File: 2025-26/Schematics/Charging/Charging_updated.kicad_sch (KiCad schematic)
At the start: 45 parts, among them J1 DTM04-12PA-L012, J10 Nema 5-20, J11 UPCR012ALS1, J12 UPCP012ALS1, J13 DTM04-12PA-L012, J14 DTM06-12SA, J2 DTM06-12SA, J20 ??? can't find PN, J3 DTM06-12SA, J4 DTM04-12PA-L012, J5 UPCP012ALS2, J6 UPCR012ALS1, J7 DTM04-12PA-L012, J8 DTM06-12SA, J9 J1772, K1 GV24 1BAX, K2 Relay_DPST-NO, K3 P115 BDA, K4 GV24 1BAX, SW1 84-5330.0020, SW2 reset, U12 IMD, U16 Battery Pack, U18 BMS, U19 DS18B20-PAR, U2 Relay board, U20 RSB, U4 6.6kW Elcon Charger, U5 Volt_indic, U6 precharge

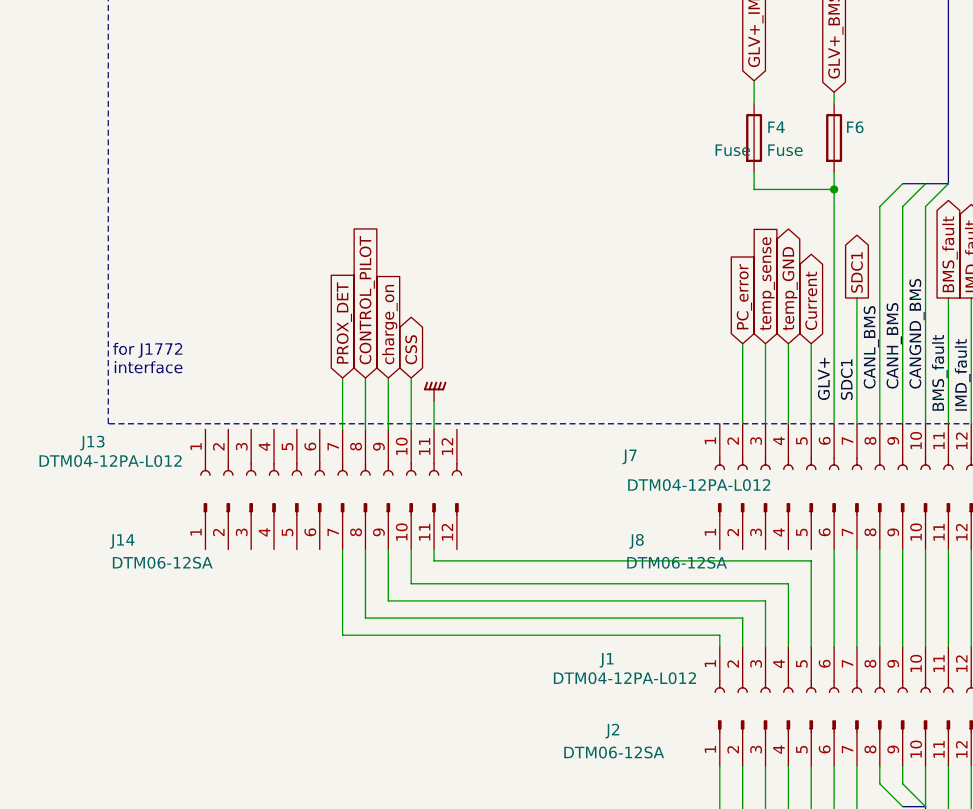
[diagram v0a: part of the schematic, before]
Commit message: Precharge and schematic updates
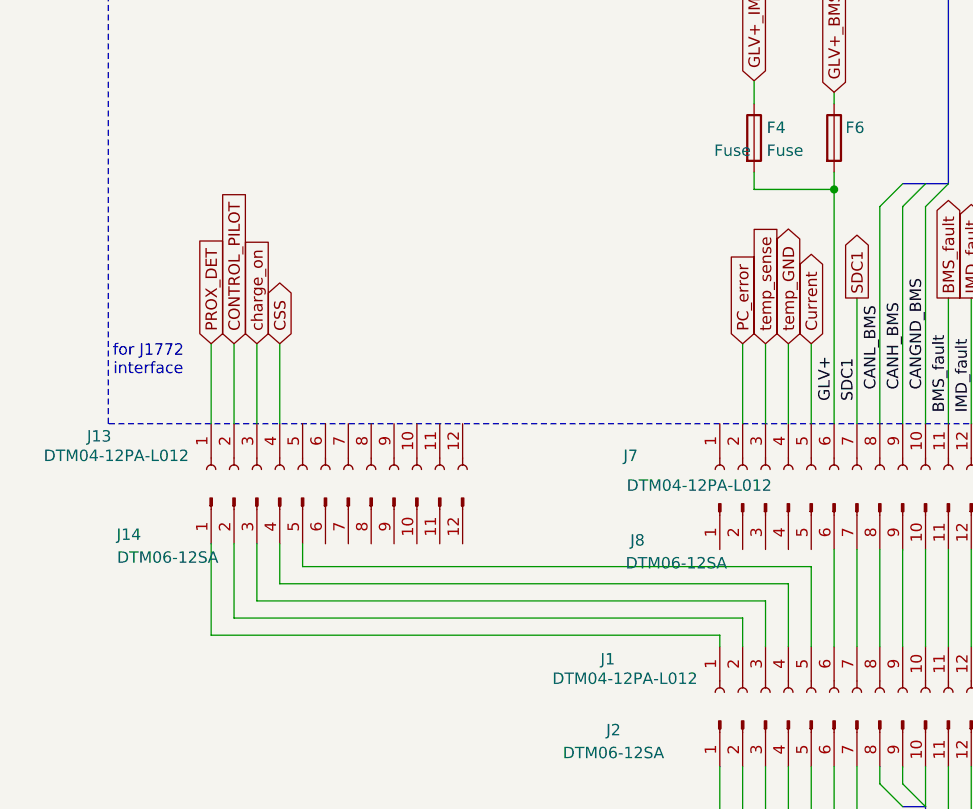
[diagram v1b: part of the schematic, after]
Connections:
- net CONTROL_PILOT: now also J13.2 (Pin_2); no longer J13.8 (Pin_8)
- net CSS: now also J13.4 (Pin_4); no longer J13.10 (Pin_10)
- net GNDPWR: no longer J13.11 (Pin_11)
- net PROX_DET: now also J13.1 (Pin_1); no longer J13.7 (Pin_7)
- net charge_on: now also J13.3 (Pin_3); no longer J13.9 (Pin_9)
- net at U16. (Tap3): no longer U18. (GND_Lug)
- net at J1.1 (Pin_1): now also J14.1 (Pin_1); no longer J14.7 (Pin_7)
- net at J1.2 (Pin_2): now also J14.2 (Pin_2); no longer J14.8 (Pin_8)
- net at J1.3 (Pin_3): now also J14.3 (Pin_3); no longer J14.9 (Pin_9)
- net at J1.4 (Pin_4): now also J14.4 (Pin_4); no longer J14.10 (Pin_10)
- net at J1.5 (Pin_5): now also J14.5 (Pin_5); no longer J14.11 (Pin_11)
- new net: U16. (Tap3), U18. (GND_Lug) (x4)
- now unconnected: U16. (Tap3), U16. (Tap3), U16. (Tap3)
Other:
- moved on the sheet: J13, J14
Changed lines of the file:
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@@
 	(wire
 		(pts
+			(xy 116.205 198.12) (xy 116.205 207.01)
+		)
+		(stroke
+			(width 0)
+			(type default)
+		)
+	)
+	(wire
+		(pts
 			(xy 302.895 153.67) (xy 325.755 153.67)
 		)
@@
 	(wire
 		(pts
-			(xy 135.89 220.98) (xy 135.89 226.695)
+			(xy 121.285 220.345) (xy 121.285 226.695)
 		)
 		(stroke
@@
 	(wire
 		(pts
-			(xy 180.34 224.79) (xy 138.43 224.79)
+			(xy 180.34 224.79) (xy 123.825 224.79)
 		)
 		(stroke
@@
 	(wire
 		(pts
-			(xy 140.97 204.47) (xy 140.97 207.645)
-		)
-		(stroke
-			(width 0)
-			(type default)
-		)
-	)
-	(wire
-		(pts
 			(xy 195.58 284.48) (xy 195.58 313.69)
 		)
@@
 	(wire
 		(pts
-			(xy 130.81 220.98) (xy 130.81 230.505)
+			(xy 116.205 220.345) (xy 116.205 230.505)
 		)
 		(stroke
@@
 	(wire
 		(pts
-			(xy 138.43 201.93) (xy 138.43 207.645)
-		)
-		(stroke
-			(width 0)
-			(type default)
-		)
-	)
-	(wire
-		(pts
 			(xy 253.365 95.885) (xy 270.51 95.885)
 		)
@@
 	(wire
 		(pts
-			(xy 175.26 228.6) (xy 133.35 228.6)
+			(xy 175.26 228.6) (xy 118.745 228.6)
 		)
 		(stroke
@@
 	(wire
 		(pts
-			(xy 138.43 220.98) (xy 138.43 224.79)
+			(xy 123.825 220.345) (xy 123.825 224.79)
 		)
 		(stroke
@@
 	(wire
 		(pts
-			(xy 140.97 220.98) (xy 140.97 222.25)
+			(xy 126.365 220.345) (xy 126.365 222.885)
 		)
 		(stroke
@@
 	(wire
 		(pts
+			(xy 118.745 198.12) (xy 118.745 207.01)
+		)
+		(stroke
+			(width 0)
+			(type default)
+		)
+	)
+	(wire
+		(pts
 			(xy 178.435 48.26) (xy 179.07 48.26)
 		)
@@
 	(wire
 		(pts
-			(xy 133.35 201.93) (xy 133.35 207.645)
-		)
-		(stroke
-			(width 0)
-			(type default)
-		)
-	)
-	(wire
-		(pts
 			(xy 180.34 284.48) (xy 180.34 287.02)
 		)
@@
 	(wire
 		(pts
+			(xy 123.825 198.12) (xy 123.825 207.01)
+		)
+		(stroke
+			(width 0)
+			(type default)
+		)
+	)
+	(wire
+		(pts
 			(xy 172.72 230.505) (xy 172.72 231.775)
 		)
@@
 	(wire
 		(pts
-			(xy 140.97 222.25) (xy 182.88 222.25)
+			(xy 126.365 222.885) (xy 182.88 222.885)
 		)
 		(stroke
@@
 	(wire
 		(pts
+			(xy 121.285 198.12) (xy 121.285 207.01)
+		)
+		(stroke
+			(width 0)
+			(type default)
+		)
+	)
+	(wire
+		(pts
 			(xy 204.47 88.9) (xy 204.47 63.5)
 		)
@@
 	(wire
 		(pts
-			(xy 135.89 201.93) (xy 135.89 207.645)
-		)
-		(stroke
-			(width 0)
-			(type default)
-		)
-	)
-	(wire
-		(pts
 			(xy 375.92 97.79) (xy 384.81 97.79)
 		)
@@
 	(wire
 		(pts
-			(xy 130.81 201.93) (xy 130.81 207.645)
-		)
-		(stroke
-			(width 0)
-			(type default)
-		)
-	)
-	(wire
-		(pts
 			(xy 393.065 374.65) (xy 395.605 374.65)
 		)
@@
 	(wire
 		(pts
-			(xy 135.89 226.695) (xy 177.8 226.695)
+			(xy 121.285 226.695) (xy 177.8 226.695)
 		)
 		(stroke
@@
 	(wire
 		(pts
-			(xy 182.88 222.25) (xy 182.88 231.775)
+			(xy 182.88 222.885) (xy 182.88 231.775)
 		)
 		(stroke
@@
 	(wire
 		(pts
-			(xy 130.81 230.505) (xy 172.72 230.505)
+			(xy 116.205 230.505) (xy 172.72 230.505)
 		)
 		(stroke
@@
 	(wire
 		(pts
-			(xy 133.35 228.6) (xy 133.35 220.98)
+			(xy 118.745 228.6) (xy 118.745 220.345)
 		)
 		(stroke
@@
 	(global_label "charge_on"
 		(shape input)
-		(at 135.89 201.93 90)
+		(at 121.285 198.12 90)
 		(fields_autoplaced yes)
 		(effects
@@
 		)
 		(property "Intersheetrefs" "${INTERSHEET_REFS}"
-			(at 135.89 189.2688 90)
+			(at 121.285 185.4588 90)
 			(effects
 				(font
@@
 	(global_label "CONTROL_PILOT"
 		(shape input)
-		(at 133.35 201.93 90)
+		(at 118.745 198.12 90)
 		(fields_autoplaced yes)
 		(effects
@@
 		)
 		(property "Intersheetrefs" "${INTERSHEET_REFS}"
-			(at 133.35 184.249 90)
+			(at 118.745 180.439 90)
 			(effects
 				(font
@@
 	(global_label "PROX_DET"
 		(shape input)
-		(at 130.81 201.93 90)
+		(at 116.205 198.12 90)
 		(fields_autoplaced yes)
 		(effects
@@
 		)
 		(property "Intersheetrefs" "${INTERSHEET_REFS}"
-			(at 130.81 189.5106 90)
+			(at 116.205 185.7006 90)
 			(effects
 				(font
@@
 	(global_label "CSS"
 		(shape bidirectional)
-		(at 138.43 201.93 90)
+		(at 123.825 198.12 90)
 		(fields_autoplaced yes)
 		(effects
@@
 		)
 		(property "Intersheetrefs" "${INTERSHEET_REFS}"
-			(at 138.43 194.1445 90)
+			(at 123.825 190.3345 90)
 			(effects
 				(font
@@
 	(symbol
 		(lib_id "Connector:Conn_01x12_Socket")
-		(at 128.27 212.725 90)
+		(at 128.905 212.09 90)
 		(mirror x)
 		(unit 1)
@@
 		(dnp no)
 		(property "Reference" "J13"
-			(at 103.124 209.042 90)
+			(at 103.759 208.407 90)
 			(effects
 				(font
@@
 		)
 		(property "Value" "DTM04-12PA-L012"
-			(at 105.029 211.201 90)
+			(at 105.664 210.566 90)
 			(effects
 				(font
@@
 		)
 		(property "Footprint" ""
-			(at 128.27 212.725 0)
+			(at 128.905 212.09 0)
 			(effects
 				(font
@@
 		)
 		(property "Datasheet" "~"
-			(at 128.27 212.725 0)
+			(at 128.905 212.09 0)
 			(effects
 				(font
@@
 		)
 		(property "Description" ""
-			(at 128.27 212.725 0)
+			(at 128.905 212.09 0)
 			(effects
 				(font
@@
 	)
 	(symbol
-		(lib_id "power:GNDPWR")
-		(at 140.97 204.47 180)
-		(unit 1)
-		(exclude_from_sim no)
-		(in_bom yes)
-		(on_board yes)
-		(dnp no)
-		(fields_autoplaced yes)
-		(property "Reference" "#PWR09"
-			(at 140.97 199.39 0)
-			(effects
-				(font
-					(size 1.27 1.27)
-				)
-				(hide yes)
-			)
-		)
-		(property "Value" "GNDPWR"
-			(at 141.097 200.66 0)
-			(effects
-				(font
-					(size 1.27 1.27)
-				)
-				(hide yes)
-			)
-		)
-		(property "Footprint" ""
-			(at 140.97 203.2 0)
-			(effects
-				(font
-					(size 1.27 1.27)
-				)
-				(hide yes)
-			)
-		)
-		(property "Datasheet" ""
-			(at 140.97 203.2 0)
-			(effects
-				(font
-					(size 1.27 1.27)
-				)
-				(hide yes)
-			)
-		)
-		(property "Description" "Power symbol creates a global label with name \"GNDPWR\" , global ground"
-			(at 140.97 204.47 0)
-			(effects
-				(font
-					(size 1.27 1.27)
-				)
-				(hide yes)
-			)
-		)
-		(pin "1"
-		)
-		(instances
-			(project "Charging_updated"
-				(path "/37f4dd62-26e6-4f3a-ae02-c1fd86435617"
-					(reference "#PWR09")
-					(unit 1)
-				)
-			)
-		)
-	)
-	(symbol
 		(lib_id "Connector:Conn_01x04_Socket")
 		(at 221.615 106.68 0)
@@
 	(symbol
 		(lib_id "Connector:Conn_01x12_Pin")
-		(at 128.27 215.9 90)
+		(at 128.905 215.265 90)
 		(mirror x)
 		(unit 1)
@@
 		(dnp no)
 		(property "Reference" "J14"
-			(at 106.426 219.964 90)
+			(at 107.061 219.329 90)
 			(effects
 				(font
@@
 		)
 		(property "Value" "DTM06-12SA"
-			(at 110.744 222.504 90)
+			(at 111.379 221.869 90)
 			(effects
 				(font
@@
 		)
 		(property "Footprint" ""
-			(at 128.27 215.9 0)
+			(at 128.905 215.265 0)
 			(effects
 				(font
@@
 		)
 		(property "Datasheet" "~"
-			(at 128.27 215.9 0)
+			(at 128.905 215.265 0)
 			(effects
 				(font
@@
 		)
 		(property "Description" ""
-			(at 128.27 215.9 0)
+			(at 128.905 215.265 0)
 			(effects
 				(font

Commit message: Precharge board updates and schematic changes
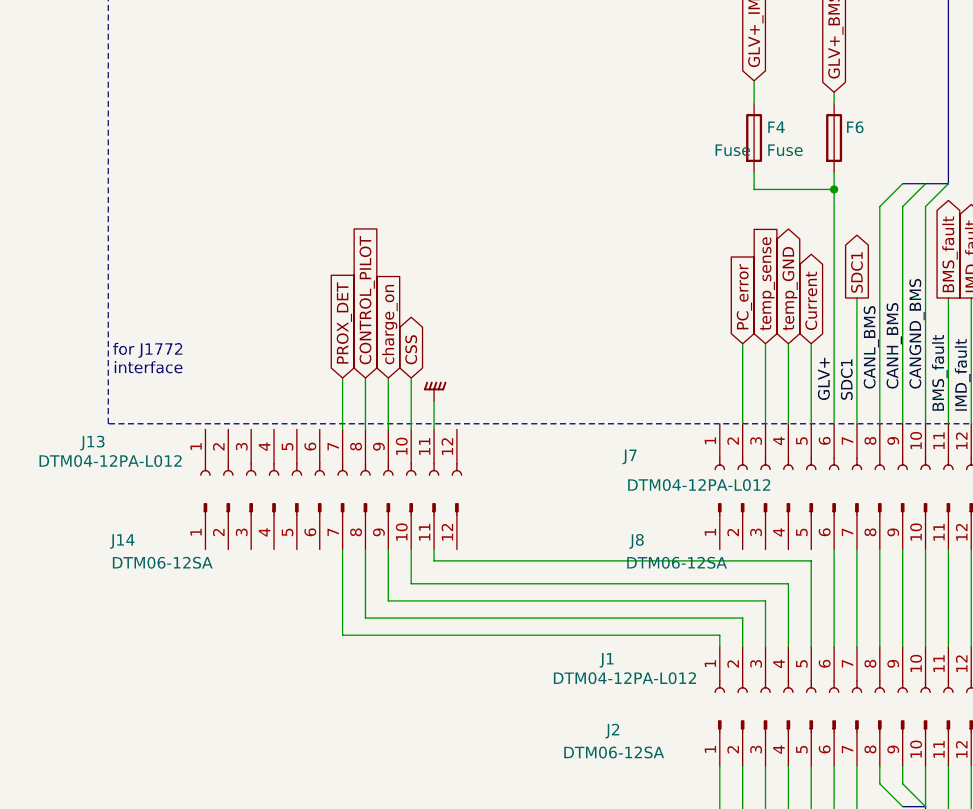
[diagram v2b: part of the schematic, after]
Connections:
- net CONTROL_PILOT: now also J13.8 (Pin_8); no longer J13.2 (Pin_2)
- net CSS: now also J13.10 (Pin_10); no longer J13.4 (Pin_4)
- net GNDPWR: now also J13.11 (Pin_11)
- net PROX_DET: now also J13.7 (Pin_7); no longer J13.1 (Pin_1)
- net charge_on: now also J13.9 (Pin_9); no longer J13.3 (Pin_3)
- net at U16. (Tap3): no longer U18. (GND_Lug)
- net at J1.1 (Pin_1): now also J14.7 (Pin_7); no longer J14.1 (Pin_1)
- net at J1.2 (Pin_2): now also J14.8 (Pin_8); no longer J14.2 (Pin_2)
- net at J1.3 (Pin_3): now also J14.9 (Pin_9); no longer J14.3 (Pin_3)
- net at J1.4 (Pin_4): now also J14.10 (Pin_10); no longer J14.4 (Pin_4)
- net at J1.5 (Pin_5): now also J14.11 (Pin_11); no longer J14.5 (Pin_5)
- new net: U16. (Tap3), U18. (GND_Lug) (x4)
- now unconnected: U16. (Tap3), U16. (Tap3), U16. (Tap3)
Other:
- moved on the sheet: J13, J14
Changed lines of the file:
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@@
 	(wire
 		(pts
-			(xy 116.205 198.12) (xy 116.205 207.01)
-		)
-		(stroke
-			(width 0)
-			(type default)
-		)
-	)
-	(wire
-		(pts
 			(xy 302.895 153.67) (xy 325.755 153.67)
 		)
@@
 	(wire
 		(pts
-			(xy 121.285 220.345) (xy 121.285 226.695)
+			(xy 135.89 220.98) (xy 135.89 226.695)
 		)
 		(stroke
@@
 	(wire
 		(pts
-			(xy 180.34 224.79) (xy 123.825 224.79)
+			(xy 180.34 224.79) (xy 138.43 224.79)
 		)
 		(stroke
@@
 	(wire
 		(pts
+			(xy 140.97 204.47) (xy 140.97 207.645)
+		)
+		(stroke
+			(width 0)
+			(type default)
+		)
+	)
+	(wire
+		(pts
 			(xy 195.58 284.48) (xy 195.58 313.69)
 		)
@@
 	(wire
 		(pts
-			(xy 116.205 220.345) (xy 116.205 230.505)
+			(xy 130.81 220.98) (xy 130.81 230.505)
 		)
 		(stroke
@@
 	(wire
 		(pts
+			(xy 138.43 201.93) (xy 138.43 207.645)
+		)
+		(stroke
+			(width 0)
+			(type default)
+		)
+	)
+	(wire
+		(pts
 			(xy 253.365 95.885) (xy 270.51 95.885)
 		)
@@
 	(wire
 		(pts
-			(xy 175.26 228.6) (xy 118.745 228.6)
+			(xy 175.26 228.6) (xy 133.35 228.6)
 		)
 		(stroke
@@
 	(wire
 		(pts
-			(xy 123.825 220.345) (xy 123.825 224.79)
+			(xy 138.43 220.98) (xy 138.43 224.79)
 		)
 		(stroke
@@
 	(wire
 		(pts
-			(xy 126.365 220.345) (xy 126.365 222.885)
+			(xy 140.97 220.98) (xy 140.97 222.25)
 		)
 		(stroke
@@
 	(wire
 		(pts
-			(xy 118.745 198.12) (xy 118.745 207.01)
-		)
-		(stroke
-			(width 0)
-			(type default)
-		)
-	)
-	(wire
-		(pts
 			(xy 178.435 48.26) (xy 179.07 48.26)
 		)
@@
 	(wire
 		(pts
+			(xy 133.35 201.93) (xy 133.35 207.645)
+		)
+		(stroke
+			(width 0)
+			(type default)
+		)
+	)
+	(wire
+		(pts
 			(xy 180.34 284.48) (xy 180.34 287.02)
 		)
@@
 	(wire
 		(pts
-			(xy 123.825 198.12) (xy 123.825 207.01)
-		)
-		(stroke
-			(width 0)
-			(type default)
-		)
-	)
-	(wire
-		(pts
 			(xy 172.72 230.505) (xy 172.72 231.775)
 		)
@@
 	(wire
 		(pts
-			(xy 126.365 222.885) (xy 182.88 222.885)
+			(xy 140.97 222.25) (xy 182.88 222.25)
 		)
 		(stroke
@@
 	(wire
 		(pts
-			(xy 121.285 198.12) (xy 121.285 207.01)
-		)
-		(stroke
-			(width 0)
-			(type default)
-		)
-	)
-	(wire
-		(pts
 			(xy 204.47 88.9) (xy 204.47 63.5)
 		)
@@
 	(wire
 		(pts
+			(xy 135.89 201.93) (xy 135.89 207.645)
+		)
+		(stroke
+			(width 0)
+			(type default)
+		)
+	)
+	(wire
+		(pts
 			(xy 375.92 97.79) (xy 384.81 97.79)
 		)
@@
 	(wire
 		(pts
+			(xy 130.81 201.93) (xy 130.81 207.645)
+		)
+		(stroke
+			(width 0)
+			(type default)
+		)
+	)
+	(wire
+		(pts
 			(xy 393.065 374.65) (xy 395.605 374.65)
 		)
@@
 	(wire
 		(pts
-			(xy 121.285 226.695) (xy 177.8 226.695)
+			(xy 135.89 226.695) (xy 177.8 226.695)
 		)
 		(stroke
@@
 	(wire
 		(pts
-			(xy 182.88 222.885) (xy 182.88 231.775)
+			(xy 182.88 222.25) (xy 182.88 231.775)
 		)
 		(stroke
@@
 	(wire
 		(pts
-			(xy 116.205 230.505) (xy 172.72 230.505)
+			(xy 130.81 230.505) (xy 172.72 230.505)
 		)
 		(stroke
@@
 	(wire
 		(pts
-			(xy 118.745 228.6) (xy 118.745 220.345)
+			(xy 133.35 228.6) (xy 133.35 220.98)
 		)
 		(stroke
@@
 	(global_label "charge_on"
 		(shape input)
-		(at 121.285 198.12 90)
+		(at 135.89 201.93 90)
 		(fields_autoplaced yes)
 		(effects
@@
 		)
 		(property "Intersheetrefs" "${INTERSHEET_REFS}"
-			(at 121.285 185.4588 90)
+			(at 135.89 189.2688 90)
 			(effects
 				(font
@@
 	(global_label "CONTROL_PILOT"
 		(shape input)
-		(at 118.745 198.12 90)
+		(at 133.35 201.93 90)
 		(fields_autoplaced yes)
 		(effects
@@
 		)
 		(property "Intersheetrefs" "${INTERSHEET_REFS}"
-			(at 118.745 180.439 90)
+			(at 133.35 184.249 90)
 			(effects
 				(font
@@
 	(global_label "PROX_DET"
 		(shape input)
-		(at 116.205 198.12 90)
+		(at 130.81 201.93 90)
 		(fields_autoplaced yes)
 		(effects
@@
 		)
 		(property "Intersheetrefs" "${INTERSHEET_REFS}"
-			(at 116.205 185.7006 90)
+			(at 130.81 189.5106 90)
 			(effects
 				(font
@@
 	(global_label "CSS"
 		(shape bidirectional)
-		(at 123.825 198.12 90)
+		(at 138.43 201.93 90)
 		(fields_autoplaced yes)
 		(effects
@@
 		)
 		(property "Intersheetrefs" "${INTERSHEET_REFS}"
-			(at 123.825 190.3345 90)
+			(at 138.43 194.1445 90)
 			(effects
 				(font
@@
 	(symbol
 		(lib_id "Connector:Conn_01x12_Socket")
-		(at 128.905 212.09 90)
+		(at 128.27 212.725 90)
 		(mirror x)
 		(unit 1)
@@
 		(dnp no)
 		(property "Reference" "J13"
-			(at 103.759 208.407 90)
+			(at 103.124 209.042 90)
 			(effects
 				(font
@@
 		)
 		(property "Value" "DTM04-12PA-L012"
-			(at 105.664 210.566 90)
+			(at 105.029 211.201 90)
 			(effects
 				(font
@@
 		)
 		(property "Footprint" ""
-			(at 128.905 212.09 0)
+			(at 128.27 212.725 0)
 			(effects
 				(font
@@
 		)
 		(property "Datasheet" "~"
-			(at 128.905 212.09 0)
+			(at 128.27 212.725 0)
 			(effects
 				(font
@@
 		)
 		(property "Description" ""
-			(at 128.905 212.09 0)
+			(at 128.27 212.725 0)
 			(effects
 				(font
@@
 	)
 	(symbol
+		(lib_id "power:GNDPWR")
+		(at 140.97 204.47 180)
+		(unit 1)
+		(exclude_from_sim no)
+		(in_bom yes)
+		(on_board yes)
+		(dnp no)
+		(fields_autoplaced yes)
+		(property "Reference" "#PWR09"
+			(at 140.97 199.39 0)
+			(effects
+				(font
+					(size 1.27 1.27)
+				)
+				(hide yes)
+			)
+		)
+		(property "Value" "GNDPWR"
+			(at 141.097 200.66 0)
+			(effects
+				(font
+					(size 1.27 1.27)
+				)
+				(hide yes)
+			)
+		)
+		(property "Footprint" ""
+			(at 140.97 203.2 0)
+			(effects
+				(font
+					(size 1.27 1.27)
+				)
+				(hide yes)
+			)
+		)
+		(property "Datasheet" ""
+			(at 140.97 203.2 0)
+			(effects
+				(font
+					(size 1.27 1.27)
+				)
+				(hide yes)
+			)
+		)
+		(property "Description" "Power symbol creates a global label with name \"GNDPWR\" , global ground"
+			(at 140.97 204.47 0)
+			(effects
+				(font
+					(size 1.27 1.27)
+				)
+				(hide yes)
+			)
+		)
+		(pin "1"
+		)
+		(instances
+			(project "Charging_updated"
+				(path "/37f4dd62-26e6-4f3a-ae02-c1fd86435617"
+					(reference "#PWR09")
+					(unit 1)
+				)
+			)
+		)
+	)
+	(symbol
 		(lib_id "Connector:Conn_01x04_Socket")
 		(at 221.615 106.68 0)
@@
 	(symbol
 		(lib_id "Connector:Conn_01x12_Pin")
-		(at 128.905 215.265 90)
+		(at 128.27 215.9 90)
 		(mirror x)
 		(unit 1)
@@
 		(dnp no)
 		(property "Reference" "J14"
-			(at 107.061 219.329 90)
+			(at 106.426 219.964 90)
 			(effects
 				(font
@@
 		)
 		(property "Value" "DTM06-12SA"
-			(at 111.379 221.869 90)
+			(at 110.744 222.504 90)
 			(effects
 				(font
@@
 		)
 		(property "Footprint" ""
-			(at 128.905 215.265 0)
+			(at 128.27 215.9 0)
 			(effects
 				(font
@@
 		)
 		(property "Datasheet" "~"
-			(at 128.905 215.265 0)
+			(at 128.27 215.9 0)
 			(effects
 				(font
@@
 		)
 		(property "Description" ""
-			(at 128.905 215.265 0)
+			(at 128.27 215.9 0)
 			(effects
 				(font
